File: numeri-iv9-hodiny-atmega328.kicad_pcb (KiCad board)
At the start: 2 copper layers, 160 x 50 mm, 64 parts, among them J2 Screw_Terminal_01x04, J3 USB-C, J4 PINHD_1x3_Female, J5 HW-084, Q1 BC557, Q2 BC557, SW1 RESET, SW2 Horizontal, SW3 Vertical, U1 ATmega328-P, U2 TPIC6B595N, U3 TPIC6B595N, U4 TPIC6B595N, U5 TPIC6B595N, Y1 6MHz

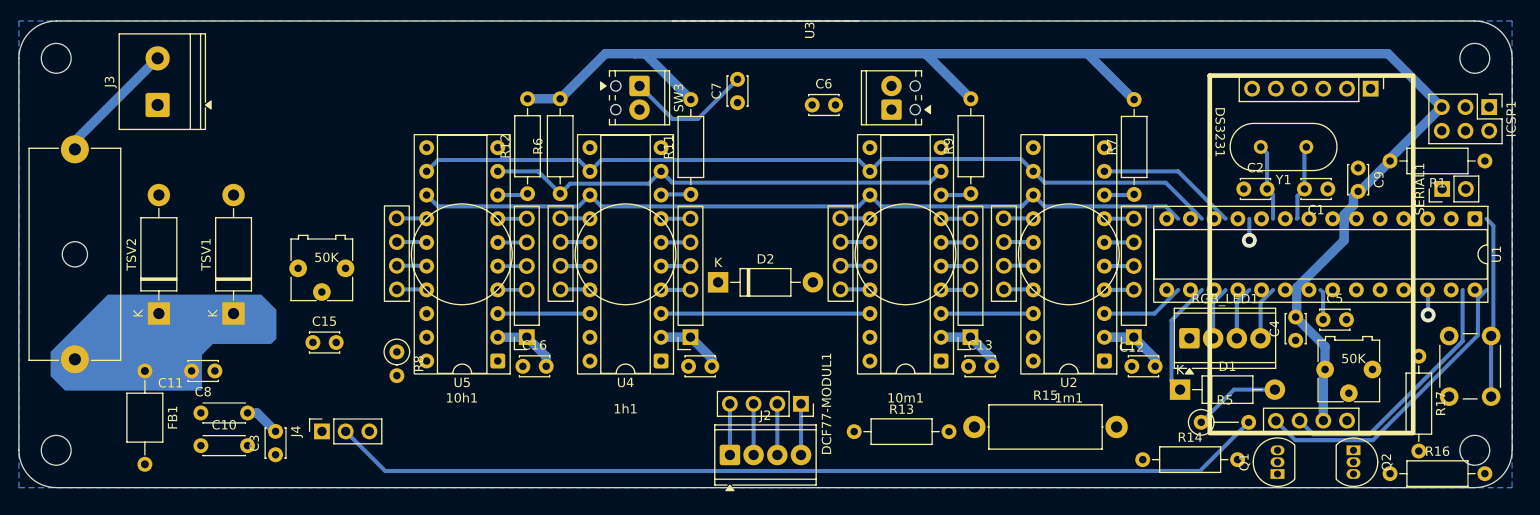
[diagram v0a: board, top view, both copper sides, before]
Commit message: preventívne
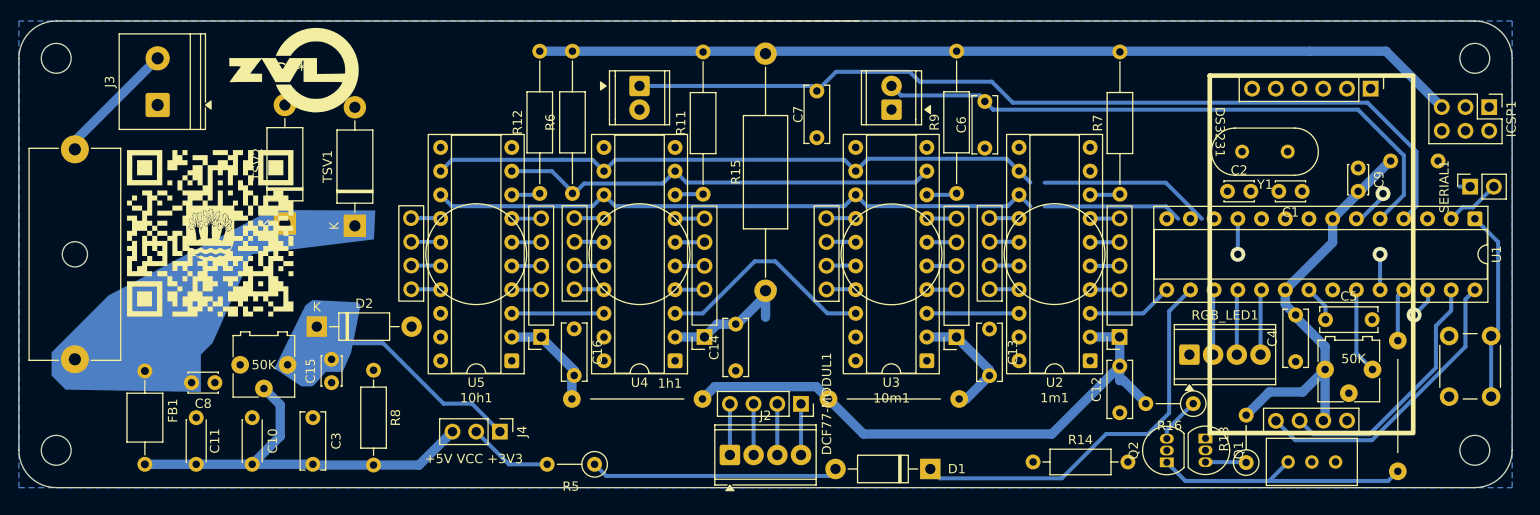
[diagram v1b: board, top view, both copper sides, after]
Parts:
- removed R17: 550R, Resistor_THT:R_Axial_DIN0207_L6.3mm_D2.5mm_P10.16mm_Horizontal
- added G***: LOGO, LOGO, F.Cu at (93.5, 75.8)
- added G***: LOGO, LOGO, F.Cu at (84.5, 93.2)
- added R4: 1K, Potentiometer_THT:Potentiometer_Bourns_3296W_Vertical, F.Cu at (200.0, 117.8)
- added REF**: JUP_P14mm, PCM_SL_Jumpers:JUP_P14mm, F.Cu at (211.8, 111.8)
- added REF**: JUP_P14mm, PCM_SL_Jumpers:JUP_P14mm, F.Cu at (130.2, 111.0)
- added REF**: JUP_P14mm, PCM_SL_Jumpers:JUP_P14mm, F.Cu at (157.8, 111.0)
- C12, C13, C14, C16, C3, C4, C5, C6, C7: footprint Capacitor_THT:C_Disc_D3.0mm_W2.0mm_P2.50mm -> Capacitor_THT:C_Disc_D6.0mm_W2.5mm_P5.00mm
- J4: footprint Connector_PinSocket_2.54mm:PinSocket_1x03_P2.54mm_Vertical -> Connector_PinHeader_2.54mm:PinHeader_1x03_P2.54mm_Vertical
- R1: footprint Resistor_THT:R_Axial_DIN0207_L6.3mm_D2.5mm_P10.16mm_Horizontal -> Resistor_THT:R_Axial_DIN0207_L6.3mm_D2.5mm_P5.08mm_Vertical; moved to B.Cu
- R11, R12, R6, R7, R9: footprint Resistor_THT:R_Axial_DIN0207_L6.3mm_D2.5mm_P10.16mm_Horizontal -> Resistor_THT:R_Axial_DIN0207_L6.3mm_D2.5mm_P15.24mm_Horizontal
- R13, R16: footprint Resistor_THT:R_Axial_DIN0207_L6.3mm_D2.5mm_P10.16mm_Horizontal -> Resistor_THT:R_Axial_DIN0207_L6.3mm_D2.5mm_P5.08mm_Vertical
- R15: footprint Resistor_THT:R_Axial_DIN0414_L11.9mm_D4.5mm_P15.24mm_Horizontal -> Resistor_THT:R_Axial_DIN0414_L11.9mm_D4.5mm_P25.40mm_Horizontal
- R8: footprint Resistor_THT:R_Axial_DIN0207_L6.3mm_D2.5mm_P2.54mm_Vertical -> Resistor_THT:R_Axial_DIN0207_L6.3mm_D2.5mm_P10.16mm_Horizontal
- SERIAL1: footprint Connector_PinHeader_2.54mm:PinHeader_1x02_P2.54mm_Vertical -> Connector_PinSocket_2.54mm:PinSocket_1x02_P2.54mm_Vertical
- SW2, SW3: footprint TerminalBlock_Phoenix:TerminalBlock_Phoenix_MPT-0,5-2-2.54_1x02_P2.54mm_Horizontal -> TerminalBlock_Phoenix:TerminalBlock_Phoenix_MPT-0,5-2-2.54_1x02_P2.54mm_Horizontal_RAW
- U2, U3, U4, U5: footprint Package_DIP:DIP-20_W7.62mm_Socket -> Package_DIP:DIP-20_W7.62mm_Socket_With_IC
- moved R5 65.2 mm to (125.7, 118.0), turned to 180 degrees
- moved D2 43.3 mm to (95.9, 103.2)
- moved R13 42.1 mm to (195.5, 117.8), turned to 90 degrees
- moved D1 28.1 mm to (161.7, 118.5), turned to 180 degrees
- moved R15 26.7 mm to (144.0, 99.4), turned to 90 degrees
- moved R16 22.4 mm to (189.8, 111.5), turned to 180 degrees
- moved Q2 20.0 mm to (187.0, 117.8), turned to 90 degrees
- moved C6 19.1 mm to (167.5, 84.1), turned to 90 degrees
- moved J4 19.1 mm to (115.5, 114.5), turned to -90 degrees
- moved TSV2 16.6 mm to (92.5, 92.2)
- moved TSV1 16.0 mm to (100.0, 92.5)
- moved RV2 12.1 mm to (90.2, 107.5)
- moved R14 11.8 mm to (172.7, 117.8)
- moved C7 9.29 mm to (149.5, 83.0)
- moved Q1 8.61 mm to (191.1, 115.2), turned to -90 degrees
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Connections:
- J4 pad 1: +3.3V -> +3V3
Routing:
- net +5V/+3V3: track 100.7 -> 9.05 mm
- net VBTN: track 13.7 -> 95.6 mm
- net +5V_DEC: track 28.8 -> 101.5 mm
- net MISO/HBTN: track 0.00 -> 66.4 mm
- net DEC_OUT: track 0.00 -> 34.6 mm
- net PB2: track 12.4 -> 43.0 mm
- net +3V3: track 0.00 -> 23.2 mm
- net +5V: track 169.7 -> 189.1 mm
- net ~{G}~: track 65.6 -> 47.5 mm
- net ~{PON}: track 9.34 -> 26.6 mm
- net Net-(U1-PC0): track 0.00 -> 9.25 mm
- net Net-(U1-XTAL2/PB7): track 8.24 -> 0.00 mm
- net Net-(U1-XTAL1/PB6): track 8.12 -> 0.00 mm
- net RX: track 0.00 -> 5.99 mm
- net Net-(Q2-E): track 0.00 -> 4.92 mm
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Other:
- board text added: "+5V VCC +3V3"
